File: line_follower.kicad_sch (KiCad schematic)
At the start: 91 parts, among them J1 Conn_01x20_Socket, J10 Conn_01x20_Pin, J11 Conn_01x20_Pin, J2 Conn_01x20_Socket, J3 Conn_01x06_Socket, J4 Conn_01x06_Socket, J5 XT60-M, J6 Conn_01x02_Socket, J7 Conn_01x02_Socket, J8 Conn_01x06_Socket, SW1 SW_Push, SW3 SW_Push, SW4 SW_Push, SW5 SW_Push

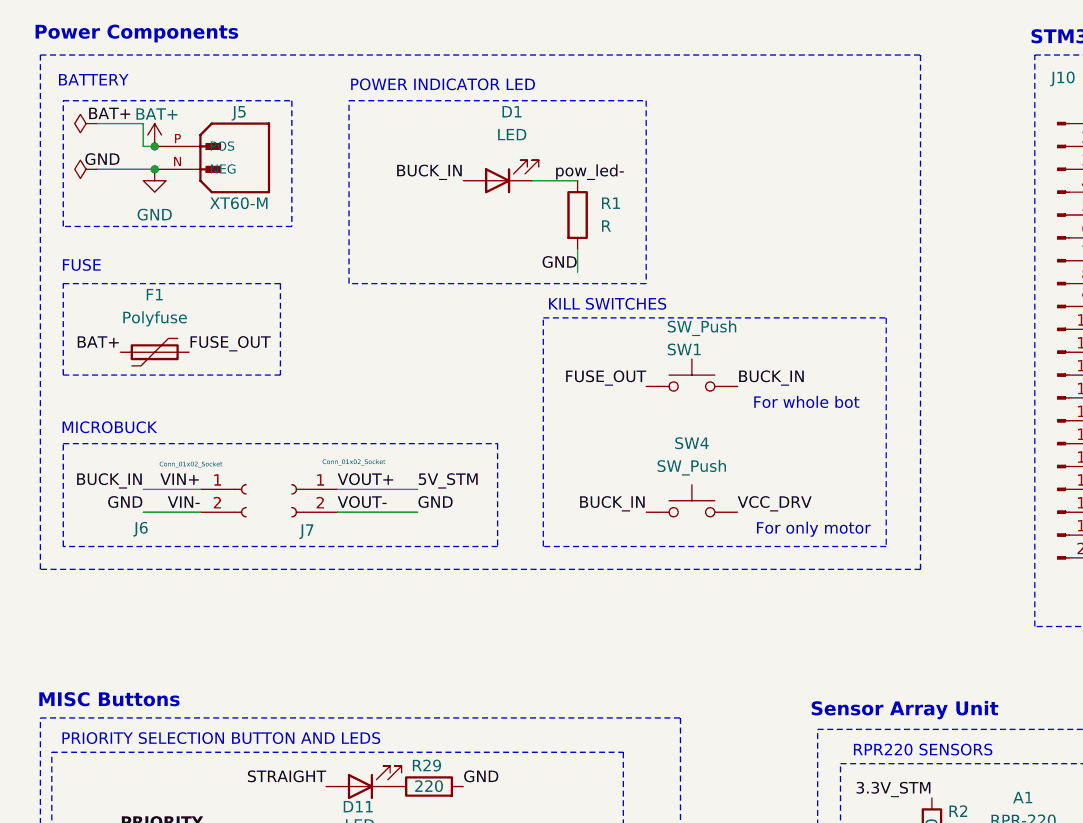
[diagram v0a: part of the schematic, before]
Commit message: schematic complete
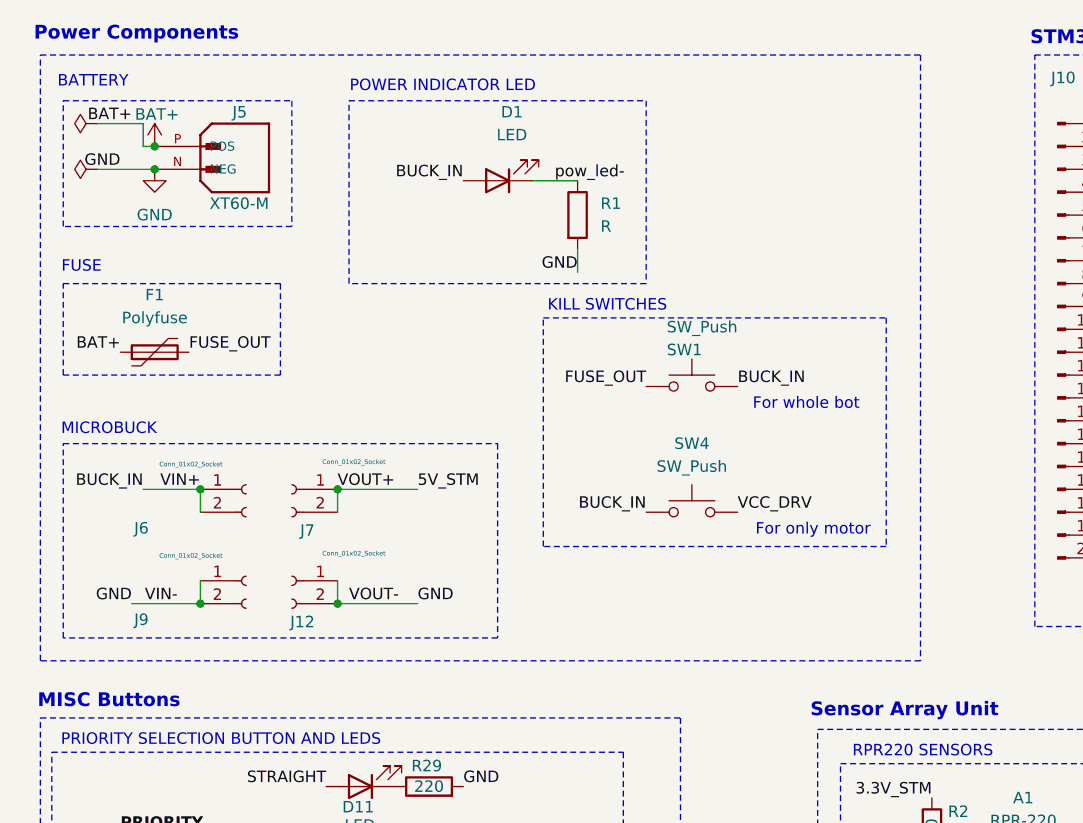
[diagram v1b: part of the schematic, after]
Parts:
- added J12, J9: Conn_01x02_Socket, Connector_PinSocket_2.54mm:PinSocket_1x02_P2.54mm_Vertical, symbol Connector:Conn_01x02_Socket
- D1, D10, D11, D12, D13, D14, D2, D3, D4, D5, D6, D7, D8, D9: footprint LED_SMD:LED_0603_1608Metric_Pad1.05x0.95mm_HandSolder -> LED_SMD:LED_0805_2012Metric_Pad1.15x1.40mm_HandSolder
- F1: footprint (none) -> Resistor_SMD:R_1812_4532Metric_Pad1.30x3.40mm_HandSolder
- J1, J2: footprint Connector_PinSocket_2.54mm:PinSocket_1x20_P2.54mm_Vertical_SMD_Pin1Left -> Connector_PinSocket_2.54mm:PinSocket_1x20_P2.54mm_Vertical
- J10, J11: footprint Connector_PinSocket_2.54mm:PinSocket_1x20_P2.54mm_Vertical_SMD_Pin1Left -> Connector_PinHeader_2.54mm:PinHeader_1x20_P2.54mm_Vertical
- J3, J4, J8: footprint Connector_PinSocket_2.54mm:PinSocket_1x06_P2.54mm_Vertical_SMD_Pin1Left -> Connector_PinSocket_2.54mm:PinSocket_1x06_P2.54mm_Vertical
- J5: footprint XT60-M:AMASS_XT60-M -> Connector_AMASS:AMASS_XT60-M_1x02_P7.20mm_Vertical
- J6, J7: footprint (none) -> Connector_PinSocket_2.54mm:PinSocket_1x02_P2.54mm_Vertical
- SW1, SW3, SW4: footprint (none) -> Button_Switch_THT:SW_Push_2P2T_Toggle_CK_PVA2xxH3xxxxxxV2
- SW5: footprint (none) -> Button_Switch_THT:SW_PUSH_6mm_H5mm
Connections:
- net 5V_STM: now also J7.2 (Pin_2)
- net BUCK_IN: now also J6.2 (Pin_2)
- net GND: now also J12.1 (Pin_1), J12.2 (Pin_2), J9.1 (Pin_1), J9.2 (Pin_2); no longer J6.2 (Pin_2), J7.2 (Pin_2)
